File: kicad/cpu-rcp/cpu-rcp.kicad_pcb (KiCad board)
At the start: 2 copper layers, 86.4 x 63.5 mm, 108 parts, among them P1 RDRAM-EDGE, P5 NINTENDO-64_PINHEAD-25X2, SW1 Reset, U1 9480F, U10 CPU-NUS, U6 PIF-NUS, U7 MX8330, U9 RCP-NUS, X1 14.318MHz

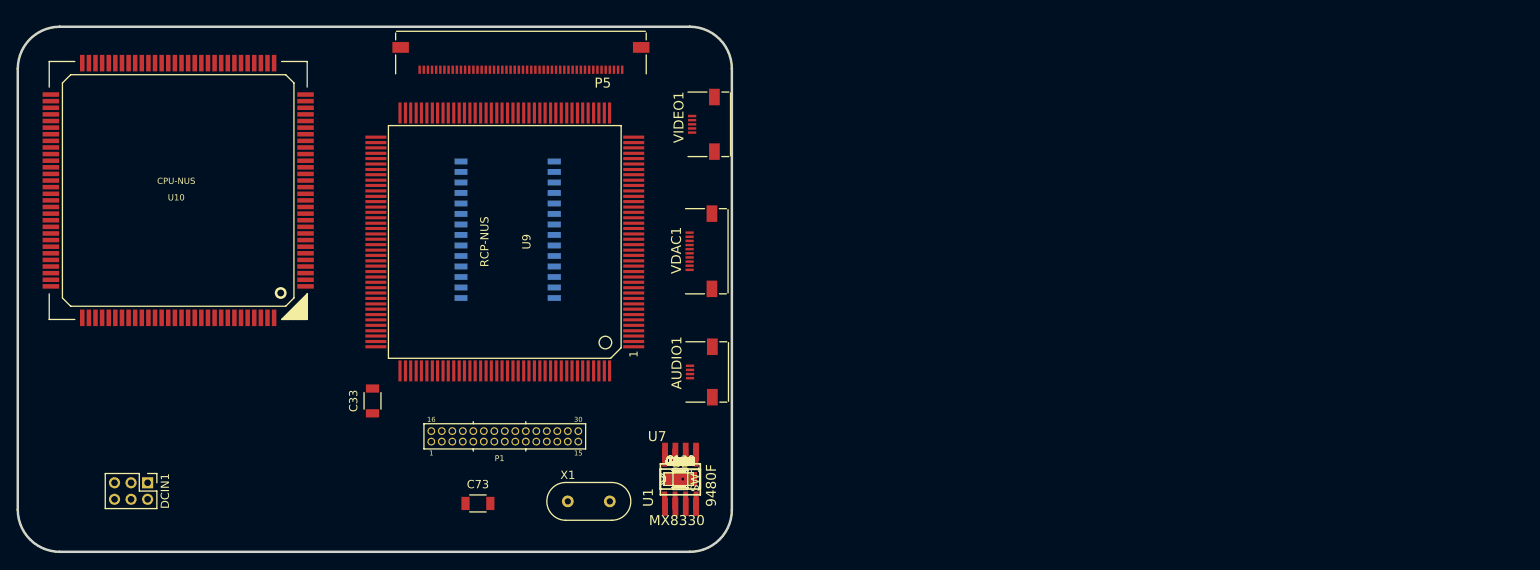
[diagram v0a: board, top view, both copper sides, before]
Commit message: Playing around
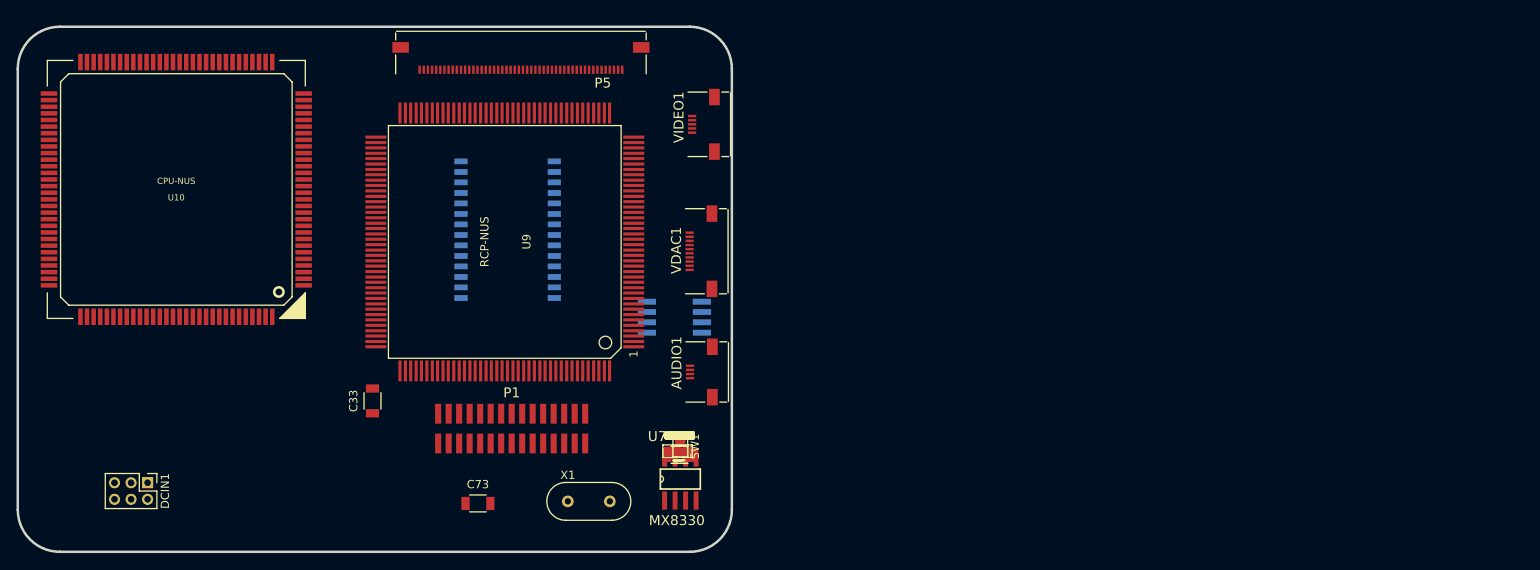
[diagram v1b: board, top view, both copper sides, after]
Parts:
- P1: footprint n64:rdram-edge -> n64:rdram-edge-smt
- U1: moved to B.Cu
- moved U1 19.6 mm to (104.8, 60.5), turned to 270 degrees
- moved P1 4.59 mm to (75.9, 71.0), turned to 0 degrees
- moved SW1 3.95 mm to (105.5, 76.2)
- moved D2 3.37 mm to (105.4, 76.7)
- moved R22 3.13 mm to (105.2, 77.0)
- moved R24 3.13 mm to (105.2, 77.0)
- moved R28 3.13 mm to (105.2, 77.0)
- moved R23 3.13 mm to (105.2, 77.0)
- moved R4 3.13 mm to (105.2, 77.0)
- moved R29 3.13 mm to (105.2, 77.0)
- moved R13 3.13 mm to (105.2, 77.0)
- moved R12 3.13 mm to (105.3, 77.0)
- moved R30 3.13 mm to (105.3, 77.0)
- moved CR19 3.13 mm to (105.3, 77.0)
- moved CR8 3.13 mm to (105.3, 77.0)
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
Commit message: Laying around, WIP
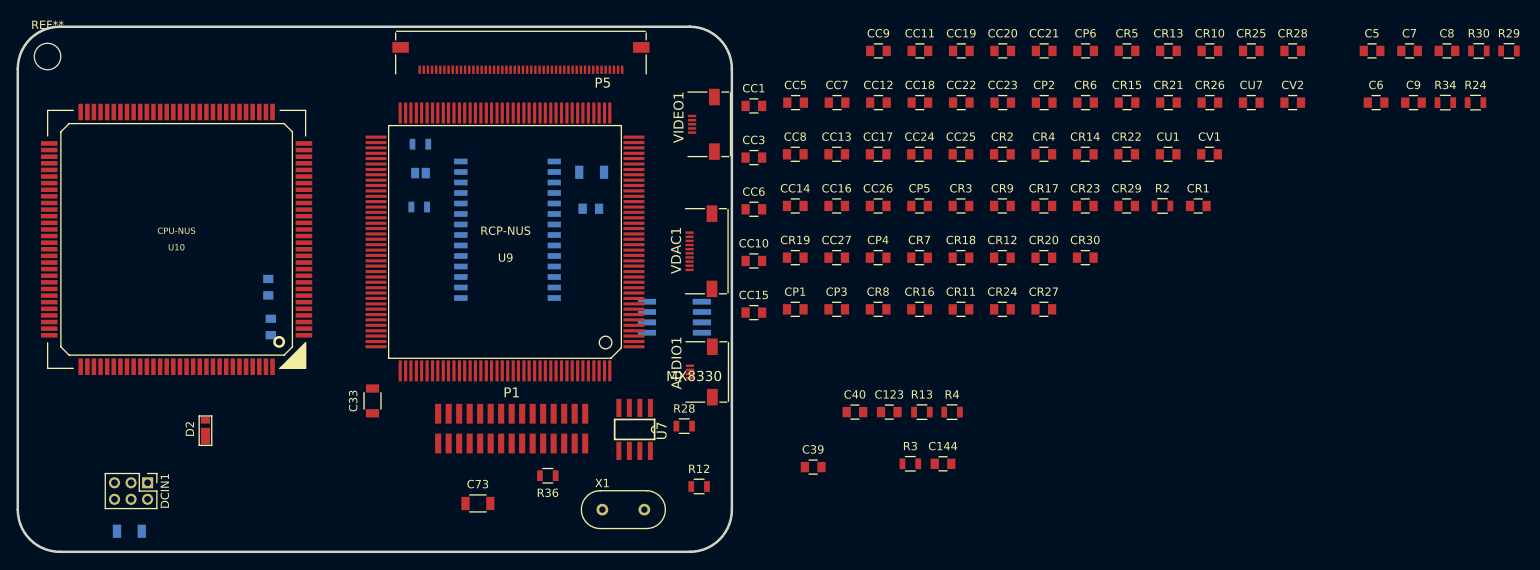
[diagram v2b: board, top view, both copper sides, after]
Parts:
- added REF**: MountingHole_3.2mm_M3, Mounting_Holes:MountingHole_3.2mm_M3_DIN965, F.Cu at (29.0, 29.0)
- C127, C128, C142, CC2, CC4, R22, R23, SW1: moved to B.Cu
- moved R29 111.7 mm to (205.7, 28.3)
- moved R30 108.4 mm to (202.1, 28.3)
- moved R24 105.4 mm to (201.7, 34.6)
- moved C8 104.8 mm to (198.2, 28.3)
- moved R34 102.0 mm to (198.0, 34.6)
- moved C7 100.8 mm to (193.7, 28.3)
- moved C9 98.4 mm to (194.2, 34.6)
- moved C5 96.9 mm to (189.2, 28.3)
- moved C6 94.3 mm to (189.7, 34.6)
- moved CR28 88.6 mm to (179.6, 28.3)
- moved CV2 85.5 mm to (179.6, 34.6)
- moved CR25 84.4 mm to (174.6, 28.3)
- moved CU7 81.1 mm to (174.6, 34.6)
- moved CR10 80.4 mm to (169.6, 28.3)
- moved CR26 76.8 mm to (169.6, 34.6)
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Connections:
- P5 pad 13: (no net) -> Net-(P5-Pad13)
- P5 pad 38: (no net) -> Net-(P5-Pad38)
- U10 pad 18: (no net) -> Net-(U10-Pad18)
- U10 pad 65: (no net) -> Net-(U10-Pad65)
- U10 pad 74: (no net) -> Net-(U10-Pad74)
- U10 pad 95: (no net) -> Net-(U10-Pad95)
- U6 pad 15: (no net) -> Net-(U6-Pad15)
- U6 pad 16: (no net) -> Net-(U6-Pad16)
- U6 pad 17: (no net) -> Net-(U6-Pad17)
- U6 pad 18: (no net) -> Net-(U6-Pad18)
- U6 pad 19: (no net) -> Net-(U6-Pad19)
- U6 pad 20: (no net) -> Net-(U6-Pad20)
- U6 pad 21: (no net) -> Net-(U6-Pad21)
- U6 pad 22: (no net) -> Net-(U6-Pad22)
- U6 pad 26: (no net) -> Net-(U6-Pad26)
- U7 pad 3: (no net) -> Net-(U7-Pad3)
